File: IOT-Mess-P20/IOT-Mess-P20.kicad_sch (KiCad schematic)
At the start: 33 parts, among them J1 Conn_01x12_Pin, J10 Jumper, J16 Jumper, J2 Conn_01x12_Pin, J3 Jumper_2, J8 Jumper, J9 Jumper, K1 Crystal, SW1 SW_Rotary_1x4_MP, SW11 SW_Push, SW2 SW_Rotary_1x6_MP, SW3 SW_Rotary_1x6_MP, SW4 SW_Rotary_1x4_MP, U10 USB_C_Receptacle_USB2.0_16P, U6 ME6211C33M5

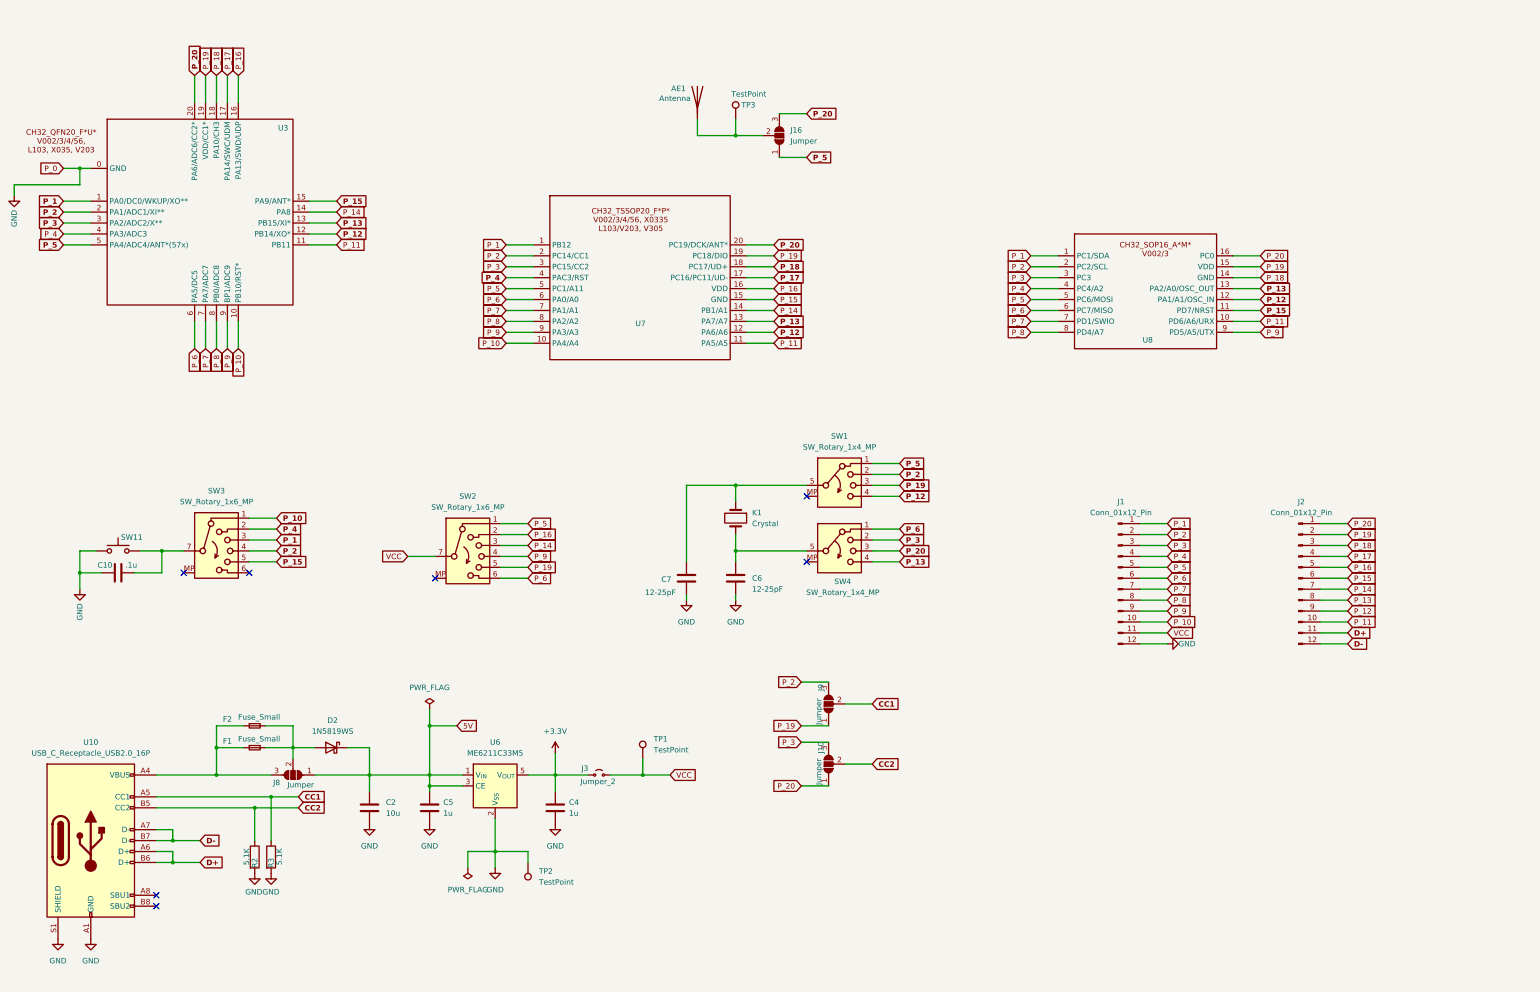
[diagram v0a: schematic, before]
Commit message: updates.
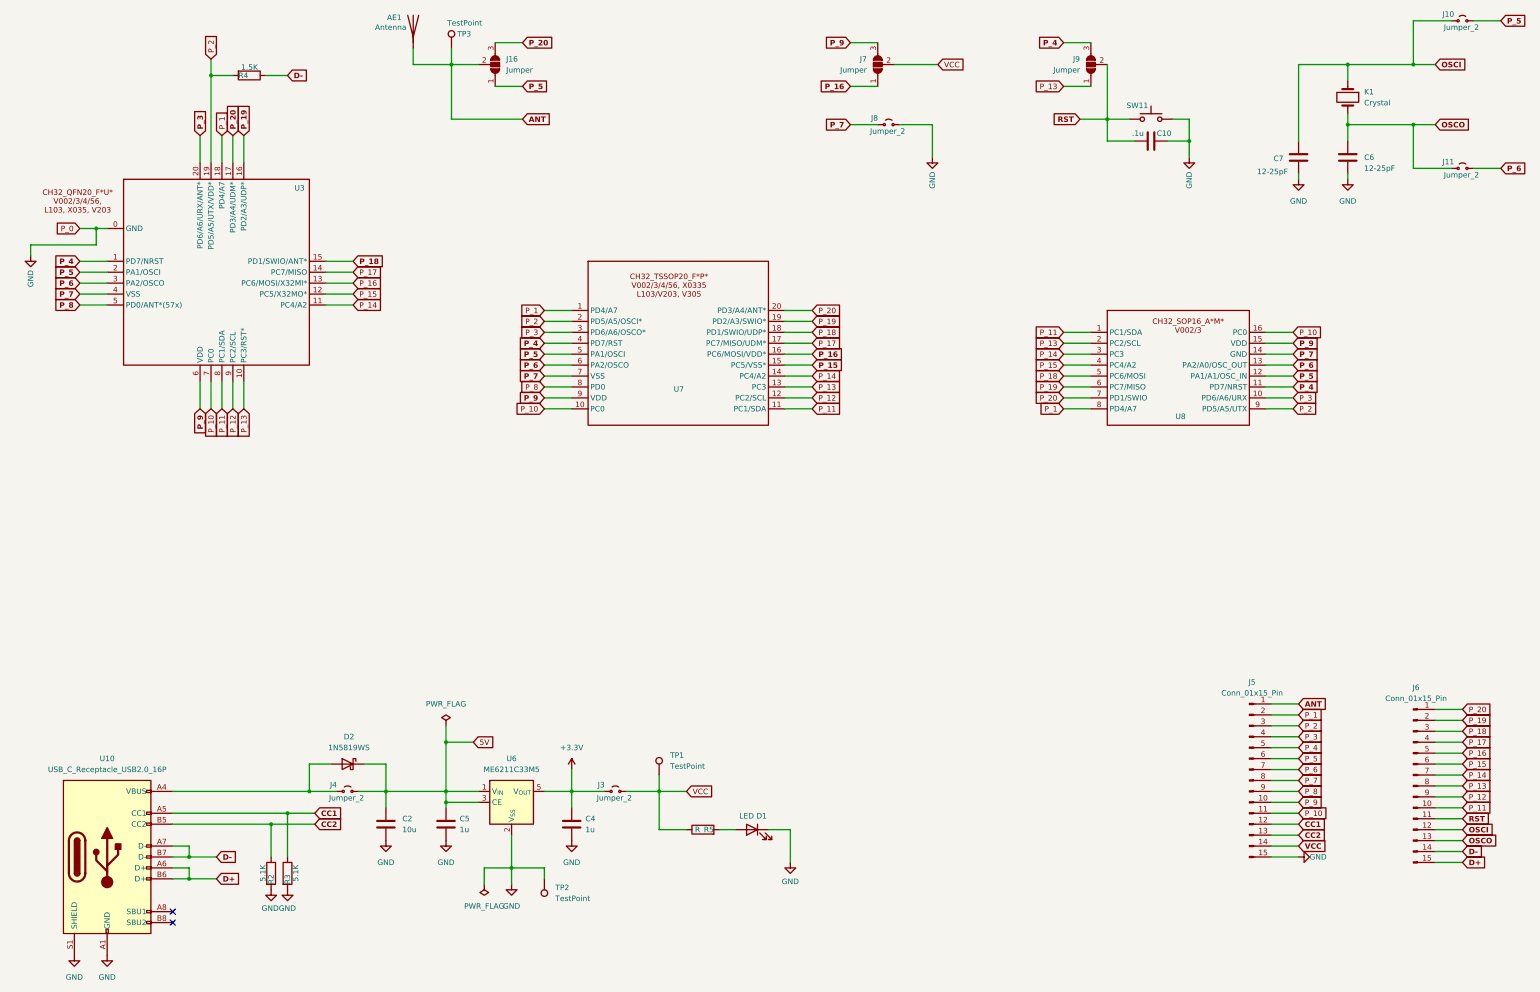
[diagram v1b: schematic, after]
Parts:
- removed F1: Fuse_Small, Fuse:Fuse_0603_1608Metric, symbol Device:Fuse_Small
- removed F2: Fuse_Small, Fuse:Fuse_0805_2012Metric, symbol Device:Fuse_Small
- removed J1, J2: Conn_01x12_Pin, Connector_PinHeader_2.54mm:PinHeader_1x12_P2.54mm_Vertical, symbol Connector:Conn_01x12_Pin
- removed J10, J8: Jumper, IOT-Mess-Footprints:Jumper-3_P1.3mm_Open_RoundedPad1.0x1.5mm, symbol Jumper:SolderJumper_3_Open
- removed SW1, SW4: SW_Rotary_1x4_MP, IOT-Mess-Footprints:Jumper4, symbol Switch:SW_Rotary_1x4_MP
- removed SW2, SW3: SW_Rotary_1x6_MP, IOT-Mess-Footprints:Jumper8, symbol Switch:SW_Rotary_1x6_MP
- added D1: LED, LED_SMD:LED_0603_1608Metric, symbol Device:LED
- added J10, J11, J4, J8: Jumper_2, IOT-Mess-Footprints:Jumpper-triangle, symbol Jumper:Jumper_2_Small_Open
- added J5, J6: Conn_01x15_Pin, Connector_PinHeader_2.54mm:PinHeader_1x15_P2.54mm_Vertical, symbol Connector:Conn_01x15_Pin
- added J7: Jumper, IOT-Mess-Footprints:Jumper-3_P1.3mm_Open_RoundedPad1.0x1.5mm, symbol Jumper:SolderJumper_3_Open
- added R4: 1.5K, Resistor_SMD:R_0603_1608Metric, symbol Device:R
- added R5: R, Resistor_SMD:R_0603_1608Metric, symbol Device:R
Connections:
- net 5V: now also J4.2 (B)
- net CC1: now also J5.12 (Pin_12); no longer J9.2 (C)
- net CC2: now also J5.13 (Pin_13)
- net D+: now also J6.15 (Pin_15)
- net D-: now also J6.14 (Pin_14), R4.1
- net GND: now also D1.1 (K), J5.15 (Pin_15), J8.2 (B)
- net P_1: now also U3.18 (PD4/A7), U8.8 (PD4/A7), J5.2 (Pin_2); no longer U3.1 (PA0/DC0/WKUP/XO**), U8.1 (PC1/SDA)
- net P_10: now also U3.7 (PC0), U8.16 (PC0), J5.11 (Pin_11); no longer U3.10 (PB10/RST*)
- net P_11: now also U3.8 (PC1/SDA), U8.1 (PC1/SDA), J6.10 (Pin_10); no longer U3.11 (PB11), U8.10 (PD6/A6/URX)
- net P_12: now also U3.9 (PC2/SCL), J6.9 (Pin_9); no longer U3.12 (PB14/XO*), U8.12 (PA1/A1/OSC_IN)
- net P_13: now also J9.1 (A), U3.10 (PC3/RST*), U8.2 (PC2/SCL), J6.8 (Pin_8); no longer U3.13 (PB15/XI*), U8.13 (PA2/A0/OSC_OUT)
- net P_14: now also U3.11 (PC4/A2), U8.3 (PC3), J6.7 (Pin_7); no longer U3.14 (PA8)
- net P_15: now also U3.12 (PC5/X32MO*), U8.4 (PC4/A2), J6.6 (Pin_6); no longer U3.15 (PA9/ANT*), U8.11 (PD7/NRST)
- net P_16: now also U3.13 (PC6/MOSI/X32MI*), J6.5 (Pin_5), J7.1 (A); no longer U3.16 (PA13/SWD/UDP)
- net P_17: now also U3.14 (PC7/MISO), J6.4 (Pin_4); no longer U3.17 (PA14/SWC/UDM)
- net P_18: now also U3.15 (PD1/SWIO/ANT*), U8.5 (PC6/MOSI), J6.3 (Pin_3); no longer U3.18 (PA10/CH3), U8.14 (GND)
- net P_19: now also U3.16 (PD2/A3/UDP*), U8.6 (PC7/MISO), J6.2 (Pin_2); no longer J9.1 (A), U3.19 (VDD/CC1*), U8.15 (VDD)
- net P_2: now also U3.19 (PD5/A5/UTX/VDD*), U8.9 (PD5/A5/UTX), J5.3 (Pin_3), R4.2; no longer J9.3 (B), U3.2 (PA1/ADC1/XI**), U8.2 (PC2/SCL)
- net P_20: now also U3.17 (PD3/A4/UDM*), U8.7 (PD1/SWIO), J6.1 (Pin_1); no longer U3.20 (PA6/ADC6/CC2*), U8.16 (PC0)
- net P_3: now also U3.20 (PD6/A6/URX/ANT*), U8.10 (PD6/A6/URX), J5.4 (Pin_4); no longer U3.3 (PA2/ADC2/X**), U8.3 (PC3)
- net P_4: now also J9.3 (B), U3.1 (PD7/NRST), U8.11 (PD7/NRST), J5.5 (Pin_5); no longer U3.4 (PA3/ADC3), U8.4 (PC4/A2)
- net P_5: now also U3.2 (PA1/OSCI), U8.12 (PA1/A1/OSC_IN), J10.2 (B), J5.6 (Pin_6); no longer U3.5 (PA4/ADC4/ANT*(57x)), U8.5 (PC6/MOSI)
- net P_6: now also U3.3 (PA2/OSCO), U8.13 (PA2/A0/OSC_OUT), J11.2 (B), J5.7 (Pin_7); no longer U3.6 (PA5/DC5), U8.6 (PC7/MISO)
- net P_7: now also U3.4 (VSS), U8.14 (GND), J5.8 (Pin_8), J8.1 (A); no longer U3.7 (PA7/ADC7), U8.7 (PD1/SWIO)
- net P_8: now also U3.5 (PD0/ANT*(57x)), J5.9 (Pin_9); no longer U3.8 (PB0/ADC8), U8.8 (PD4/A7)
- net P_9: now also U3.6 (VDD), U8.15 (VDD), J5.10 (Pin_10), J7.3 (B); no longer U3.9 (BP1/ADC9), U8.9 (PD5/A5/UTX)
- net VCC: now also J5.14 (Pin_14), J7.2 (C), R5.1
- net ANT: now reaches AE1.1 (A), J16.2 (C), TP3.1
- net ANT: now also J5.1 (Pin_1)
- net OSCI: now reaches C7.1, K1.1
- net OSCI: now also J10.1 (A), J6.12 (Pin_12)
- net at U10.A4 (VBUS), U10.A9 (VBUS), U10.B4 (VBUS)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: now also D2.2 (A), J4.1 (A)
- net OSCO: now reaches C6.1, K1.2
- net OSCO: now also J11.1 (A), J6.13 (Pin_13)
- net RST: now reaches C10.1, SW11.1
- net RST: now also J9.2 (C), J6.11 (Pin_11)
- new net: D1.2 (A), R5.2
- no-connect marks 7 -> 2
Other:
- moved on the sheet: AE1, C10, C2, C4, C5, C6, C7, D2, J16, J3, K1, R2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
